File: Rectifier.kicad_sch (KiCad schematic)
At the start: 0 parts

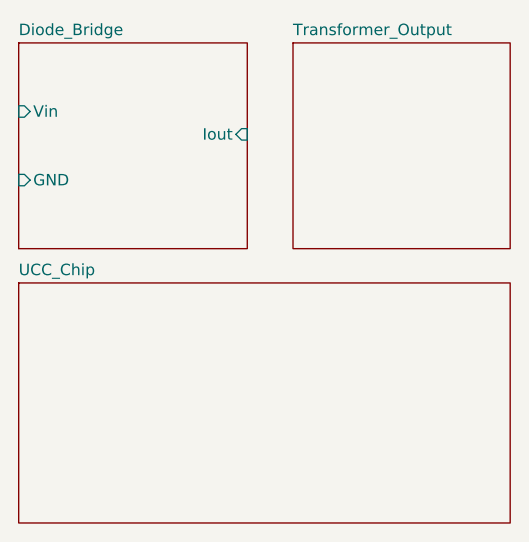
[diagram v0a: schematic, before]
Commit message: Changed Name of sheet
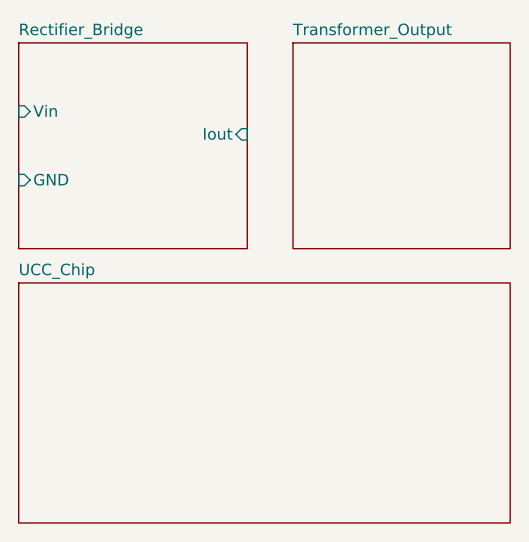
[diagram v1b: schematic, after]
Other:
- sheet Diode_Bridge renamed Rectifier_Bridge
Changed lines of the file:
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@@
 			(color 0 0 0 0)
 		)
-		(property "Sheetname" "Diode_Bridge"
+		(property "Sheetname" "Rectifier_Bridge"
 			(at 107.95 104.6984 0)
 			(show_name no)

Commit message: note
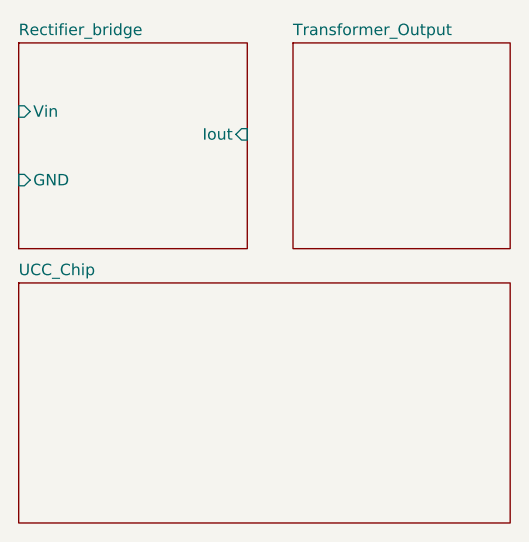
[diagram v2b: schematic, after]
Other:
- sheet Rectifier_Bridge renamed Rectifier_bridge
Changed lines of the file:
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@@
 			(color 0 0 0 0)
 		)
-		(property "Sheetname" "Rectifier_Bridge"
+		(property "Sheetname" "Rectifier_bridge"
 			(at 107.95 104.6984 0)
 			(show_name no)

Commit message: test
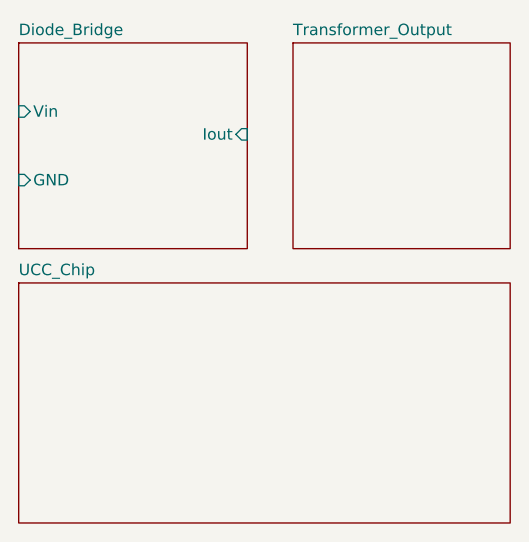
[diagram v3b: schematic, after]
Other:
- sheet Rectifier_bridge renamed Diode_Bridge
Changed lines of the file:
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@@
 			(color 0 0 0 0)
 		)
-		(property "Sheetname" "Rectifier_bridge"
+		(property "Sheetname" "Diode_Bridge"
 			(at 107.95 104.6984 0)
 			(show_name no)
